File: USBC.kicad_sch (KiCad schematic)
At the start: 4 parts, among them J2 USB_C_Receptacle_USB2.0_16P

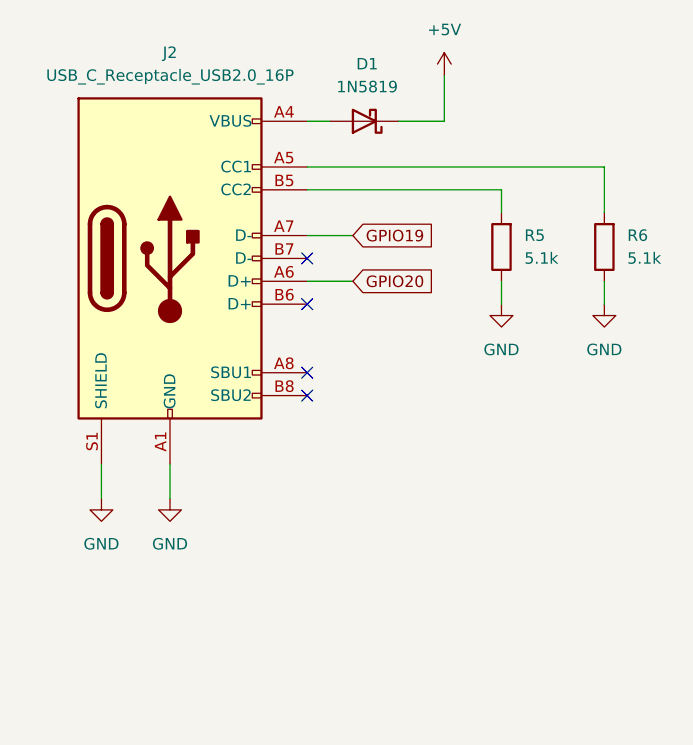
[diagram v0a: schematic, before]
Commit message: updated schematic
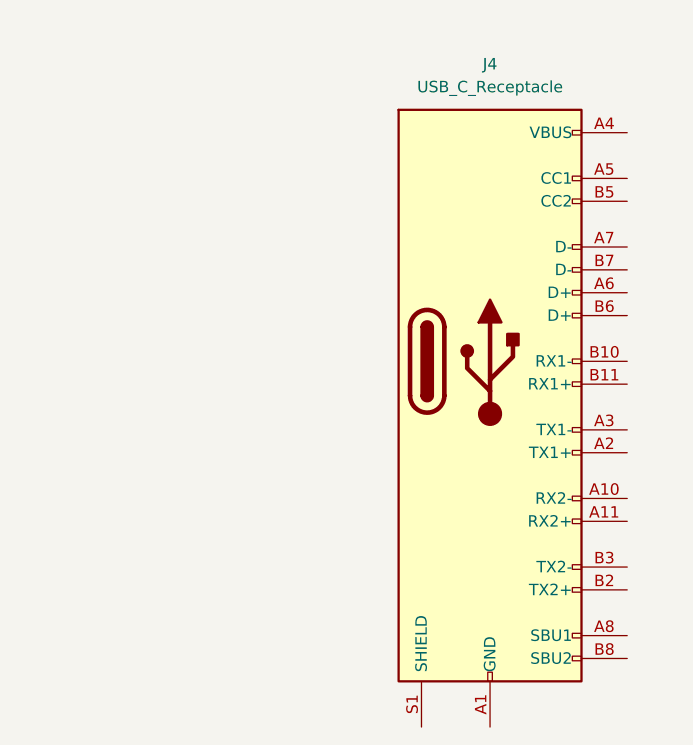
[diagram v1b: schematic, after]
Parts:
- removed D1: 1N5819, Diode_THT:D_DO-41_SOD81_P10.16mm_Horizontal, symbol Diode:1N5819
- removed J2: USB_C_Receptacle_USB2.0_16P, symbol Connector:USB_C_Receptacle_USB2.0_16P
- removed R5, R6: 5.1k, Resistor_SMD:R_0603_1608Metric_Pad0.98x0.95mm_HandSolder, symbol Device:R
- added J4: USB_C_Receptacle, symbol Connector:USB_C_Receptacle
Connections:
- new net: J4.A1 (GND), J4.A12 (GND), J4.B1 (GND), J4.B12 (GND)
- new net: J4.A4 (VBUS), J4.A9 (VBUS), J4.B4 (VBUS), J4.B9 (VBUS)
- no-connect marks 4 -> 0
